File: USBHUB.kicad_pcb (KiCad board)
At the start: 2 copper layers, 24 parts, among them J1 Screw_Terminal_01x02, J2 USB_C_Receptacle, Q1 SI3421DV, Q2 SI3421DV, U1 CYPD3177_24x

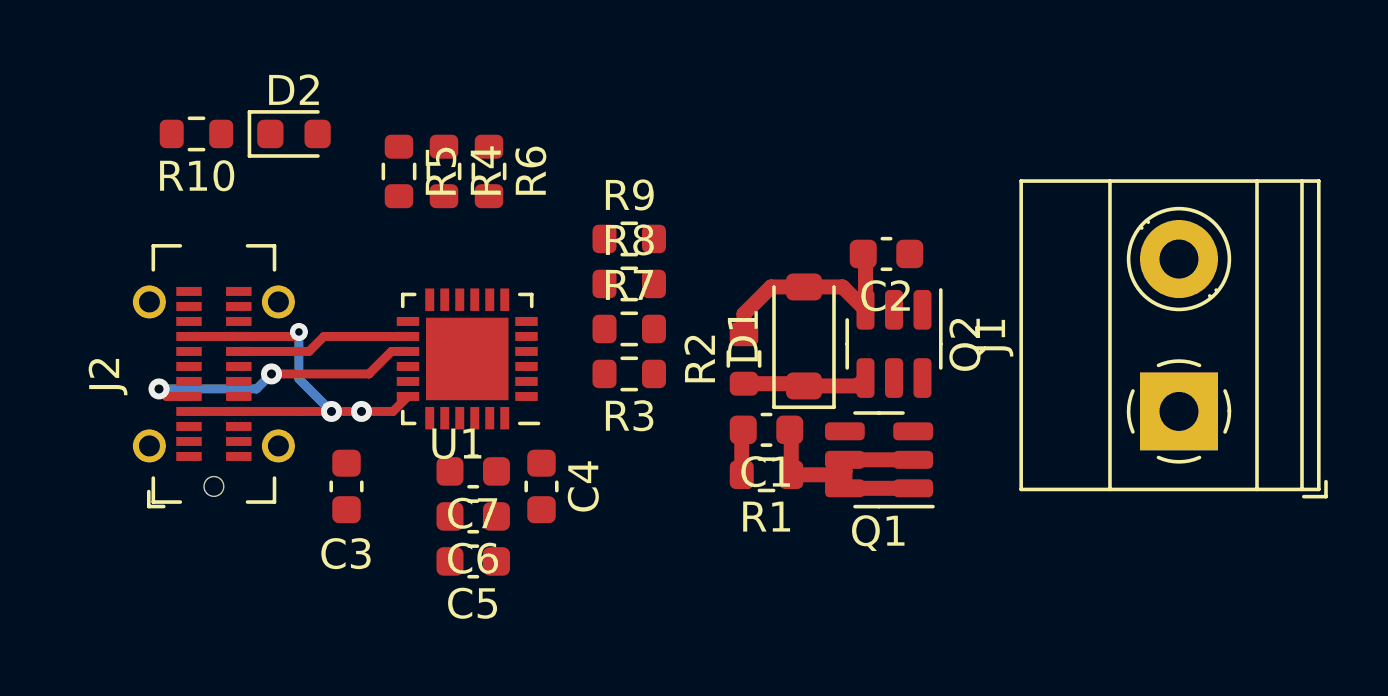
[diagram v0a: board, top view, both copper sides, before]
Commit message: Finish PCB design
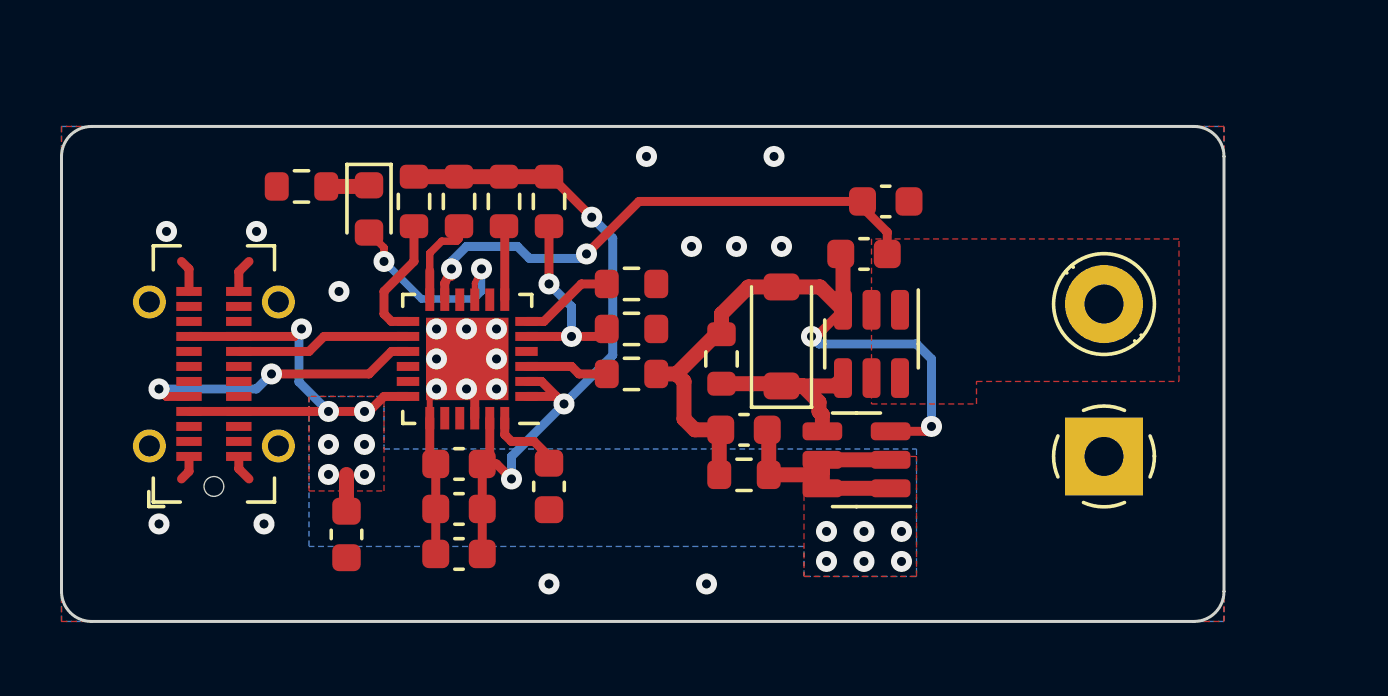
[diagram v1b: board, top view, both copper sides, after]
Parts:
- added C8: 3u3, Capacitor_SMD:C_0603_1608Metric, F.Cu at (73.0, 78.5)
- moved R10 15.3 mm to (64.5, 81.2), turned to 0 degrees
- moved R8 11.4 mm to (53.5, 78.0), turned to 180 degrees
- moved R7 5.02 mm to (61.8, 78.5), turned to -90 degrees
- moved D2 3.54 mm to (55.8, 78.8), turned to -90 degrees
- moved R9 3.00 mm to (64.5, 82.8)
- moved J1 2.92 mm to (80.2, 87.0)
- moved C3 1.60 mm to (55.0, 89.6)
- moved R4 1.12 mm to (58.8, 78.5)
- moved R5 1.12 mm to (57.2, 78.5)
- moved R6 1.12 mm to (60.2, 78.5)
- moved C1 0.75 mm to (68.2, 86.1)
- moved C2 0.75 mm to (72.2, 80.2)
- moved D1 0.75 mm to (69.5, 83.0)
- moved Q1 0.75 mm to (72.0, 87.1)
- moved Q2 0.75 mm to (72.5, 83.2)
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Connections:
- J1 pad 1: +20V -> GND
- J1 pad 2: GND -> +20V
- U1 pad 10: USB_UFP_FLIP -> unconnected-(U1-FLIP-Pad10)
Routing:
- net /USB_PD_VDDD_3V3: track 0.00 -> 26.0 mm, vias 0 -> 3
- net +20V: track 0.00 -> 18.3 mm, vias 0 -> 2
- net Net-(D1-A): track 8.83 -> 23.9 mm, vias 0 -> 2
- net GND: track 0.00 -> 11.3 mm, vias 0 -> 20
- net /FAULT: track 0.00 -> 7.12 mm, vias 0 -> 2
- net Net-(U1-ISNK_COARSE): track 0.00 -> 6.76 mm, vias 0 -> 2
- net Net-(U1-HPI_SCL): track 0.00 -> 4.24 mm
- net Net-(U1-HPI_SDA): track 0.00 -> 3.25 mm
- net Net-(U1-ISNK_FINE): track 0.00 -> 3.19 mm
- net Net-(U1-VBUS_FET_EN): track 0.00 -> 2.78 mm
- net Net-(U1-VCCD): track 0.00 -> 2.55 mm
- net Net-(D1-K): track 4.21 -> 6.70 mm
- net Net-(U1-HPI_INT): track 0.00 -> 2.46 mm
- net VBUS: track 23.2 -> 24.7 mm, vias 3 -> 13
- net Net-(D2-K): track 0.00 -> 1.44 mm
- added copper zone on F.Cu, net +20V
- added copper zone on B.Cu, net GND
- added copper zone on F.Cu, net GND
- added copper zone on B.Cu, net VBUS
- added copper zone on F.Cu, net VBUS
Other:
- board outline added: 38.8 x 16.5 mm
